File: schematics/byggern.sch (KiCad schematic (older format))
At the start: 5 parts

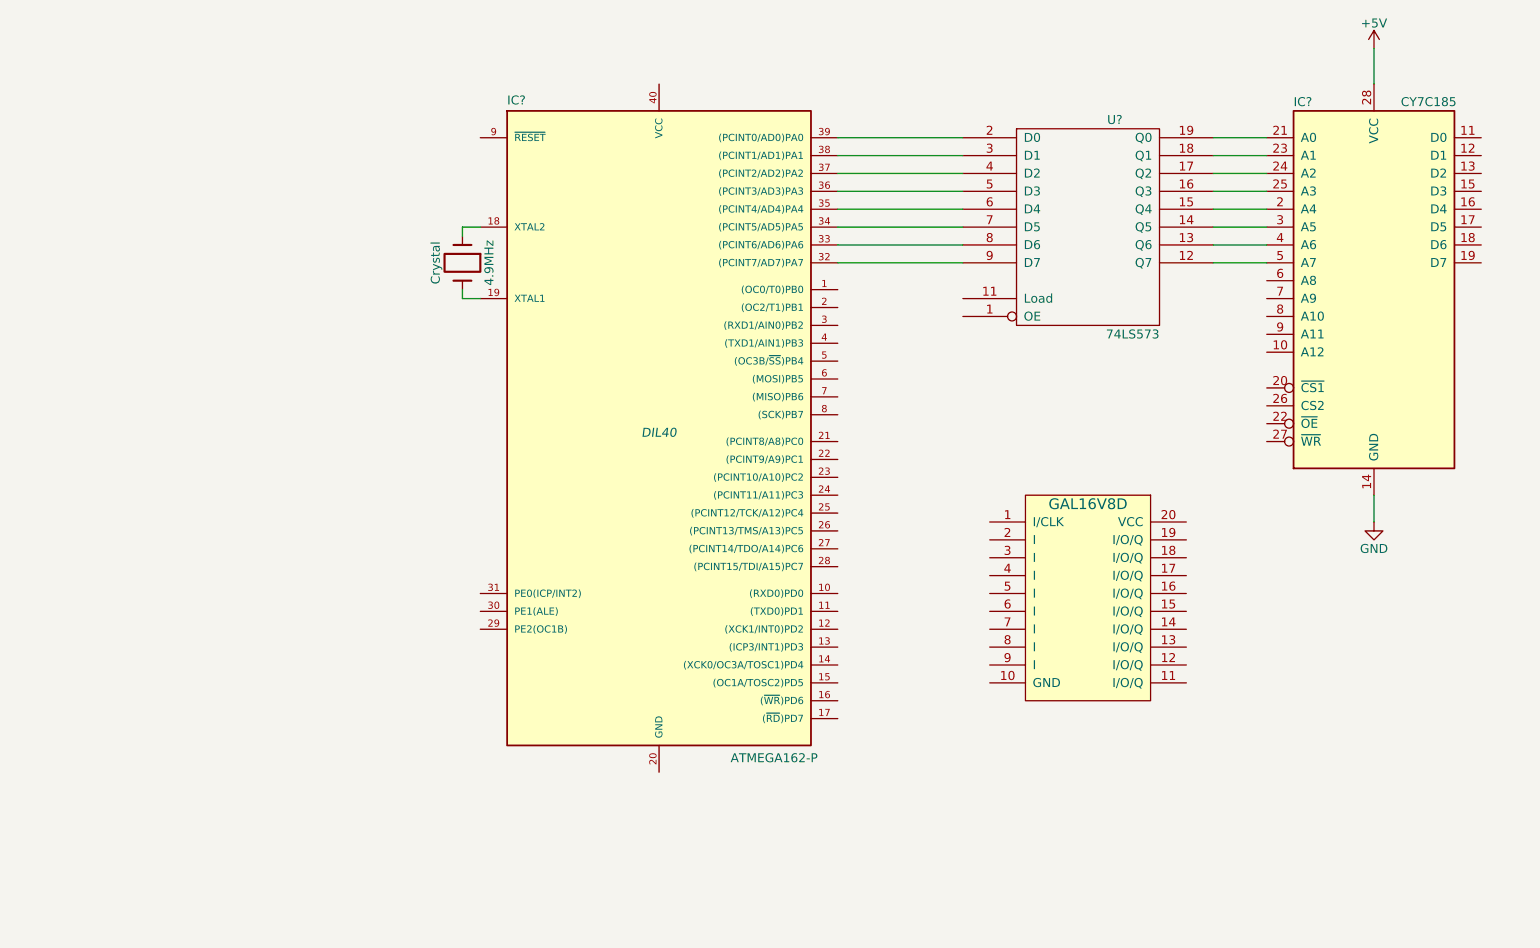
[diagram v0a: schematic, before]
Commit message: Further work on sch
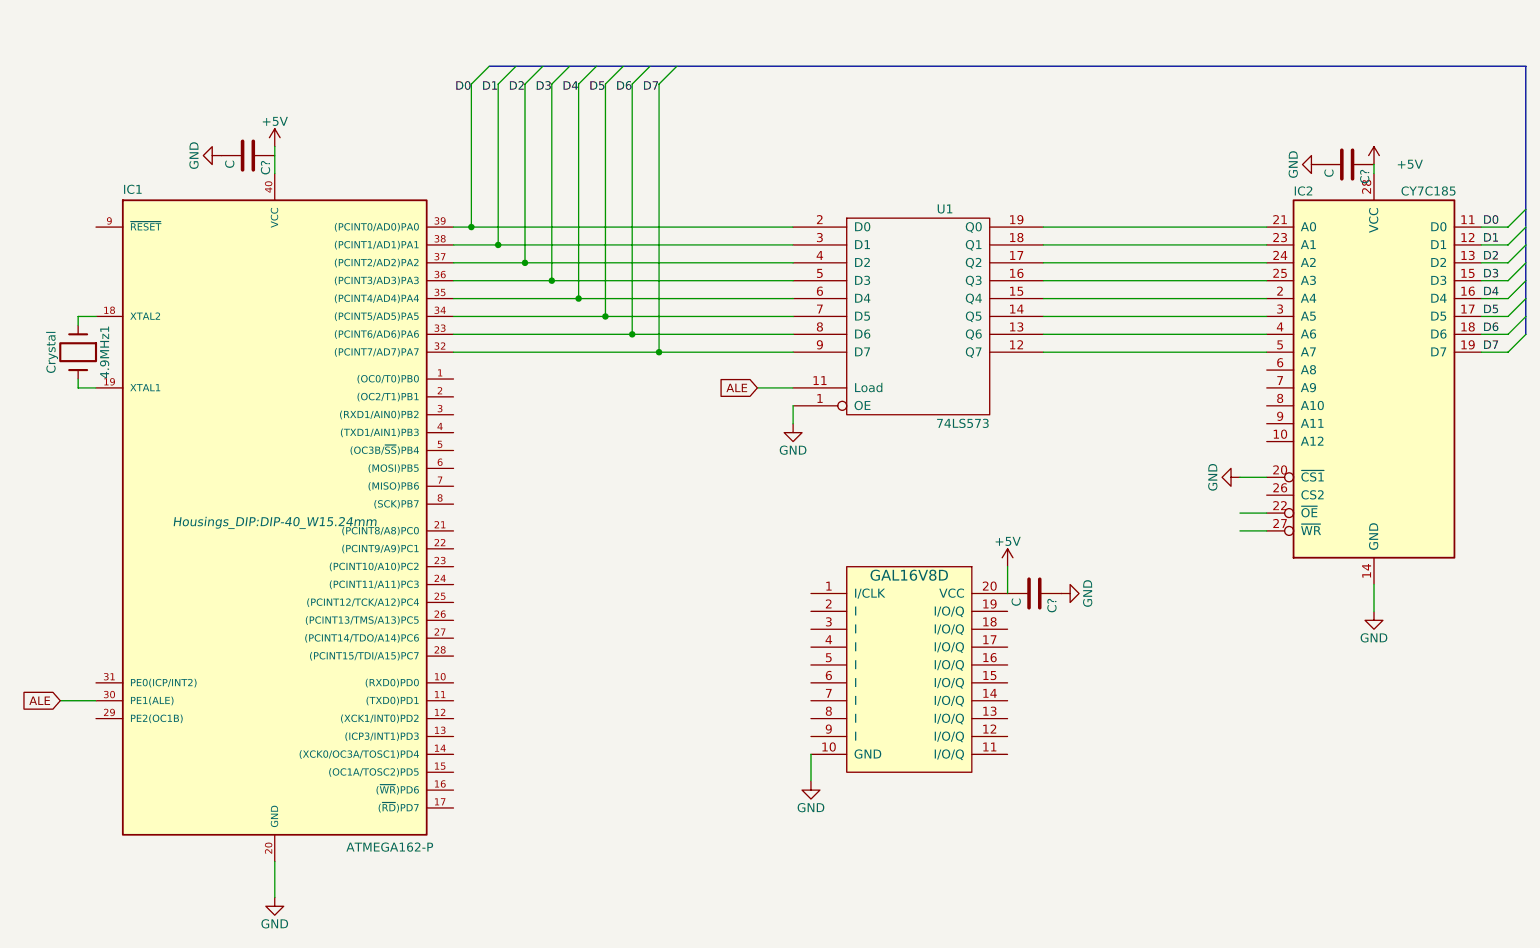
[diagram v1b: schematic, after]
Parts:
- added C? (x3): C, symbol C
- 4.9MHz1: renamed from 4.9MHz; footprint (none) -> Crystals:crystal_FA238-TSX3225
- IC1: renamed from IC?; footprint DIL40 -> Housings_DIP:DIP-40_W15.24mm
- IC2: renamed from IC?; footprint (none) -> Housings_DIP:DIP-28_W7.62mm
- U1, U2: renamed from U?; footprint (none) -> Housings_DIP:DIP-20_W7.62mm
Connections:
- net labels added: ALE, D0, D1, D2, D3, D4, D5, D6, D7
- wire segments 22 -> 48
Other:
- moved on the sheet: 4.9MHz1, IC1, IC2, U1
